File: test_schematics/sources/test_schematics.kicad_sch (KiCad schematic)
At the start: 0 parts

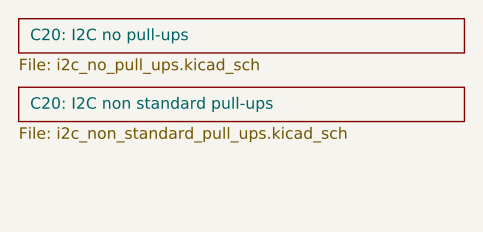
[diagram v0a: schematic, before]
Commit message: feat: basic I2C buses finder.
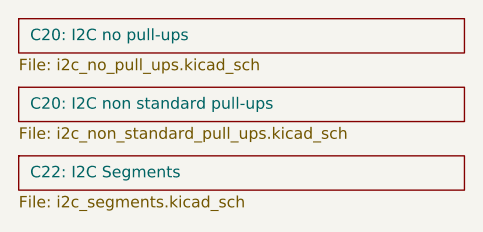
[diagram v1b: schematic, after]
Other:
- added sheet C22: I2C Segments (i2c_segments.kicad_sch)
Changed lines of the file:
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@@
+		)
+	)
+	(sheet
+		(at 13.97 31.75)
+		(size 49.53 3.81)
+		(stroke
+			(width 0.1524)
+			(type solid)
+		)
+		(fill
+			(color 0 0 0 0.0000)
+		)
+		(property "Sheetname" "C22: I2C Segments"
+			(at 15.24 34.29 0)
+			(effects
+				(font
+					(size 1.27 1.27)
+				)
+				(justify left bottom)
+			)
+		)
+		(property "Sheetfile" "i2c_segments.kicad_sch"
+			(at 13.97 36.1446 0)
+			(effects
+				(font
+					(size 1.27 1.27)
+				)
+				(justify left top)
+			)
+		)
+		(instances
+			(project "test_schematics"
+				(path "/f327a4b6-22d9-4671-bd1f-2c46b703509e"
+					(page "4")
+				)
+			)
 		)
 	)
